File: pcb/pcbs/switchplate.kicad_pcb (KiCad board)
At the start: 2 copper layers, 152.4 x 110.9 mm, 5 parts

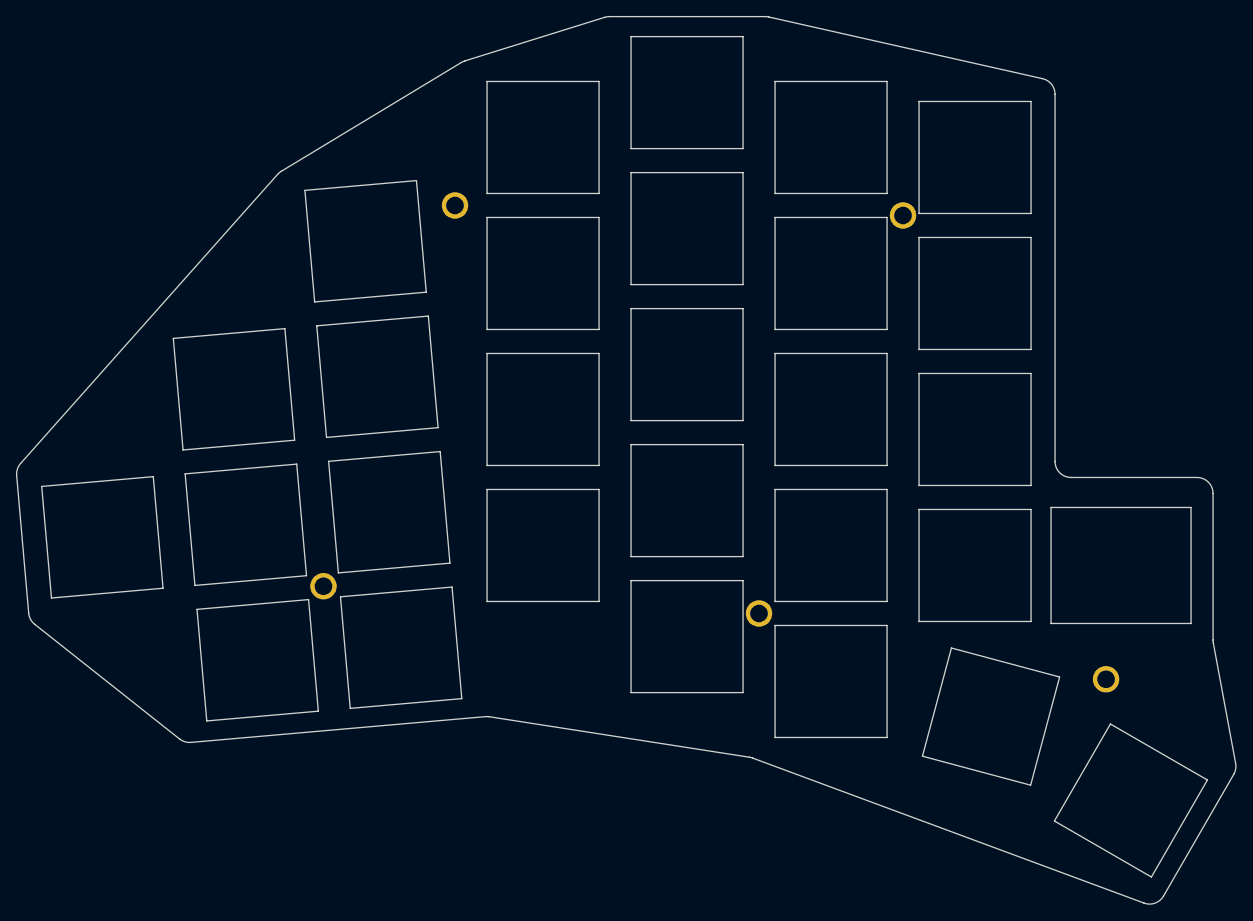
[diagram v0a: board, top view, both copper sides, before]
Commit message: kicad 7.0.6
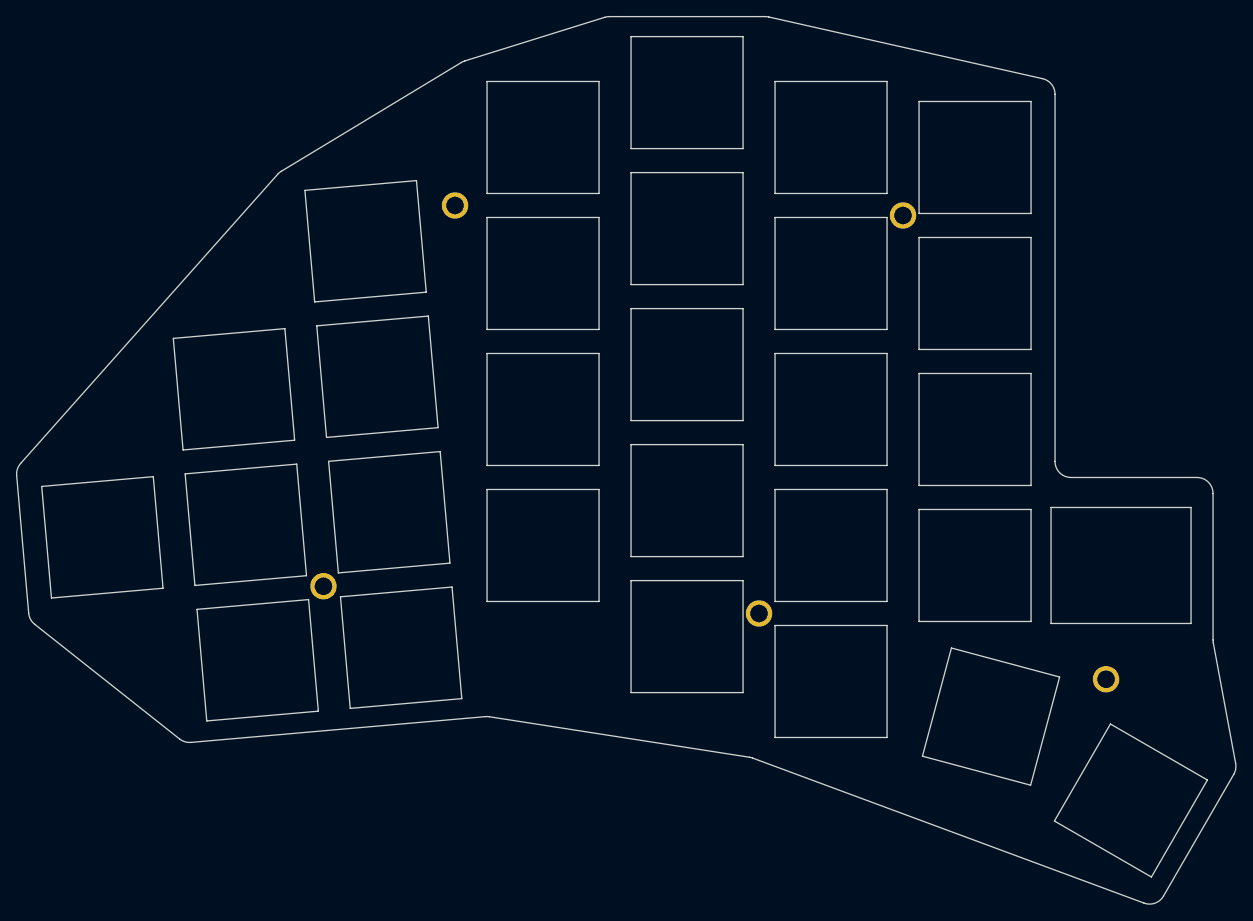
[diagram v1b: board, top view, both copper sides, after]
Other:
- net class Default removed

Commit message: switchplate distances
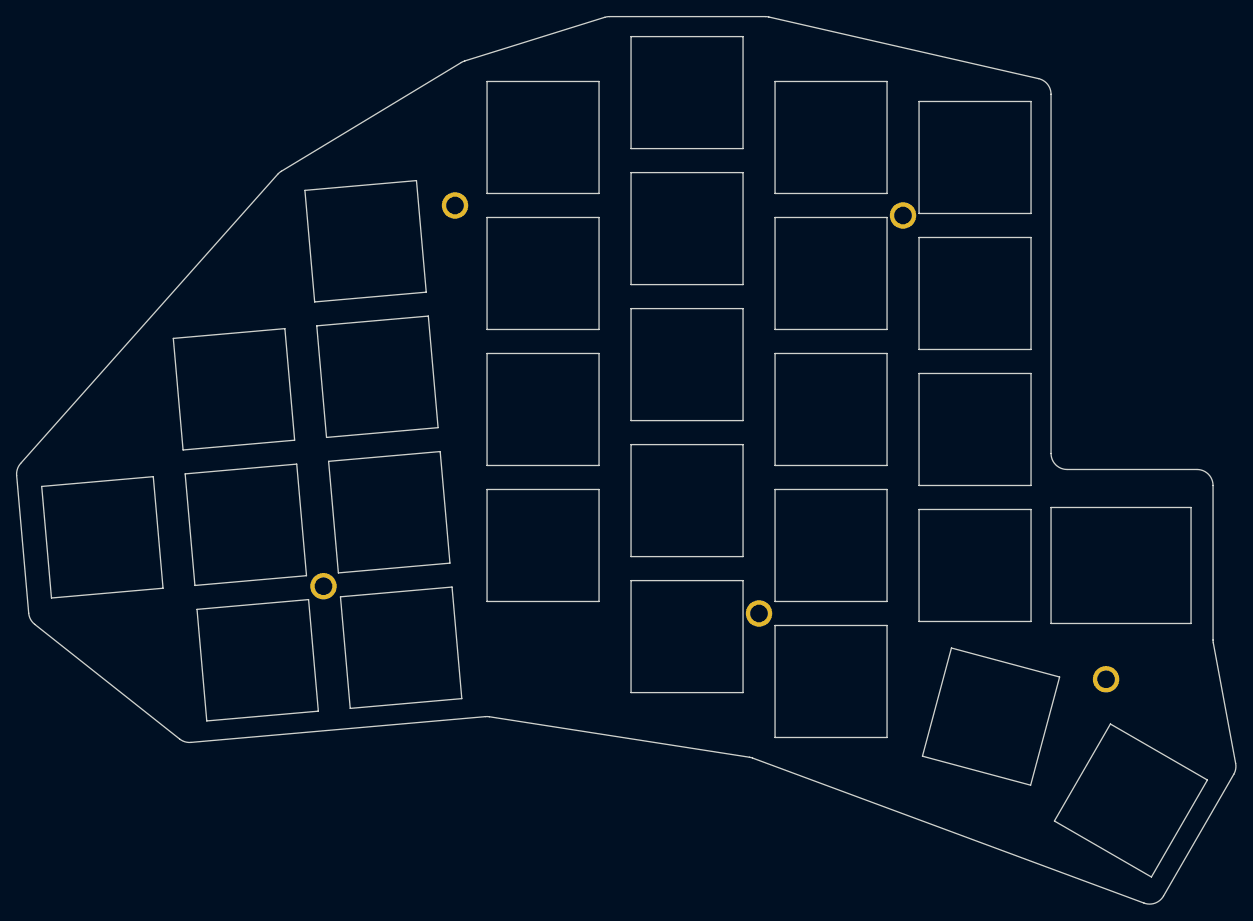
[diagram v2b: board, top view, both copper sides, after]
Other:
- outline, holes or cut-outs redrawn
- net class Default added: clearance 0.2, trace_width 0.25, via_dia 0.8, via_drill 0.4
